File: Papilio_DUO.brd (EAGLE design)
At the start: 101.6 x 55.9 mm, 125 parts, among them IC1 FT2232H, SW1 SWITCH-2CH-6P-3010010P1, SW2 EVQQ2, T100 MOSFET-NCHANNELSMD, U1 ARDUINO_MEGA_SHIELD, U100 PCA9306, U101 ATMEGA32U4-XUMU, U2 LTC3419EMS, U3 93C46B, X1 12MHz, Y1 16MHz KX-7

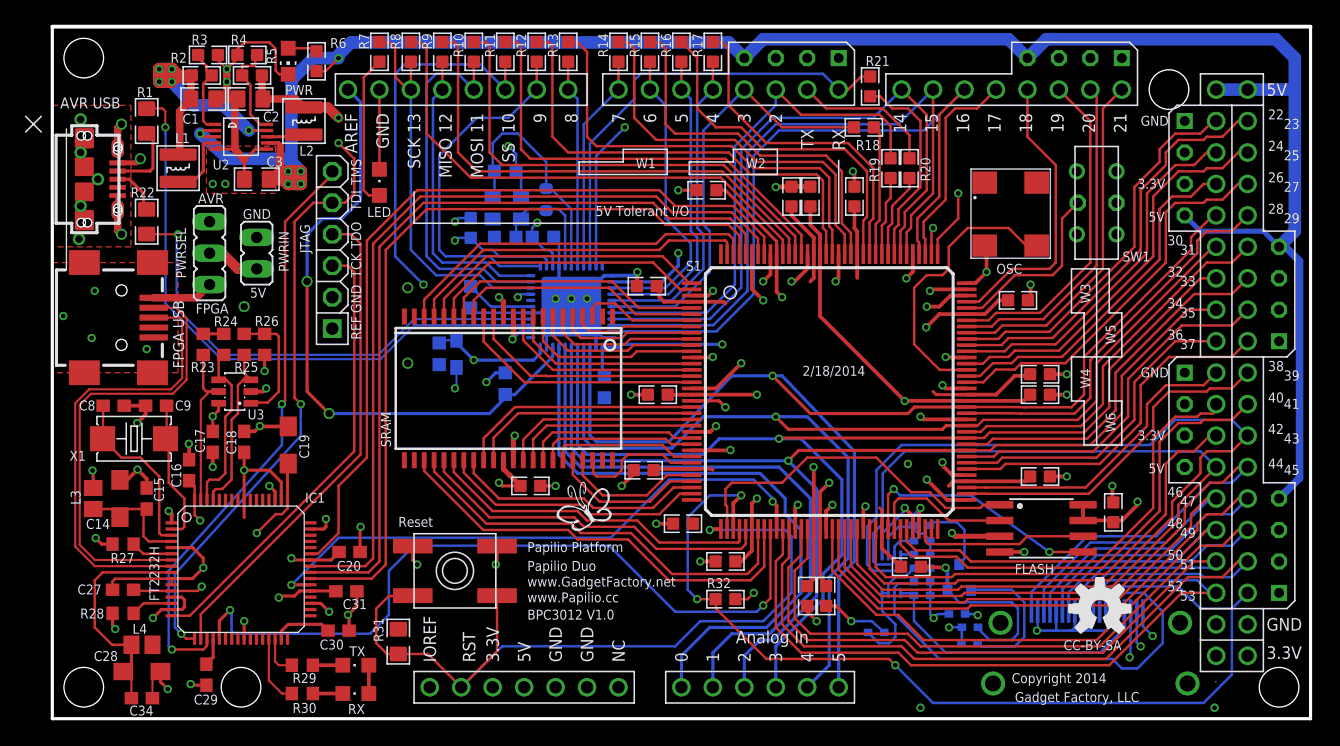
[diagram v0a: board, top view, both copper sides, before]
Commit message: Papilio DUO V1.1
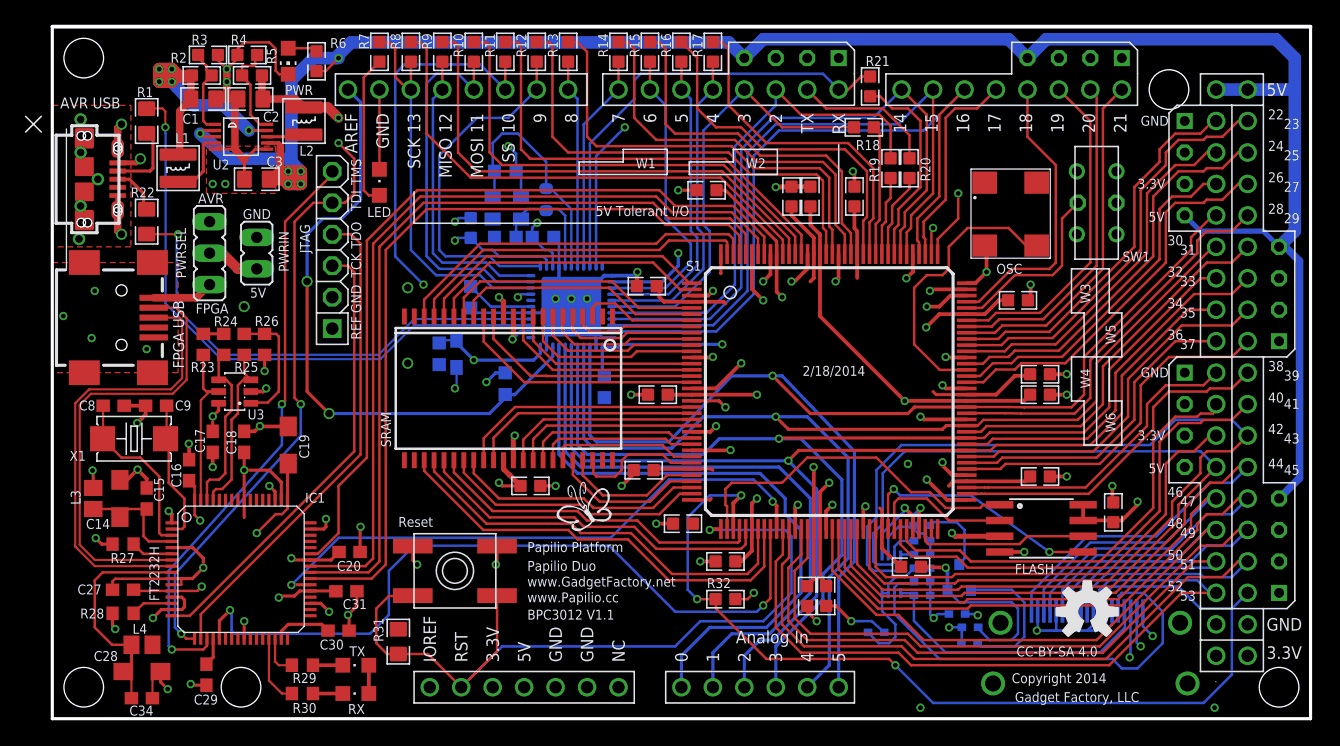
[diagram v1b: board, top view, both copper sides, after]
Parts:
- moved U$9 1.05 mm to (83.6, 8.64)
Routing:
- net 3V3: track 213.5 -> 216.7 mm
- net GND: track 237.0 -> 237.7 mm
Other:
- board text added: "BPC3012 V1.1"
- board text added: "CC-BY-SA 4.0"
- board text removed: "BPC3012 V1.0"
- board text removed: "CC-BY-SA"
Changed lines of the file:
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@@
 <setting verticaltext="up"/>
 </settings>
-<grid distance="0.05" unitdist="inch" unit="inch" style="lines" multiple="1" display="yes" altdistance="0.005" altunitdist="inch" altunit="inch"/>
+<grid distance="10" unitdist="mil" unit="mil" style="lines" multiple="1" display="yes" altdistance="1" altunitdist="mil" altunit="mil"/>
 <layers>
-<layer number="1" name="Top" color="4" fill="1" visible="yes" active="yes"/>
+<layer number="1" name="Top" color="4" fill="1" visible="no" active="yes"/>
 <layer number="2" name="Route2" color="6" fill="1" visible="no" active="yes"/>
 <layer number="3" name="Route3" color="11" fill="1" visible="no" active="yes"/>
 <layer number="14" name="Route14" color="1" fill="6" visible="no" active="no"/>
 <layer number="15" name="Route15" color="5" fill="1" visible="no" active="no"/>
-<layer number="16" name="Bottom" color="1" fill="1" visible="yes" active="yes"/>
+<layer number="16" name="Bottom" color="1" fill="1" visible="no" active="yes"/>
 <layer number="17" name="Pads" color="2" fill="1" visible="yes" active="yes"/>
 <layer number="18" name="Vias" color="2" fill="1" visible="yes" active="yes"/>
@@
 <layer number="22" name="bPlace" color="13" fill="1" visible="yes" active="yes"/>
 <layer number="23" name="tOrigins" color="15" fill="1" visible="yes" active="yes"/>
-<layer number="24" name="bOrigins" color="15" fill="1" visible="yes" active="yes"/>
+<layer number="24" name="bOrigins" color="15" fill="1" visible="no" active="yes"/>
 <layer number="25" name="tNames" color="7" fill="1" visible="yes" active="yes"/>
 <layer number="26" name="bNames" color="7" fill="1" visible="no" active="yes"/>
@@
 <layer number="29" name="tStop" color="12" fill="3" visible="no" active="yes"/>
 <layer number="30" name="bStop" color="12" fill="6" visible="no" active="yes"/>
-<layer number="31" name="tCream" color="7" fill="4" visible="no" active="yes"/>
+<layer number="31" name="tCream" color="7" fill="4" visible="yes" active="yes"/>
 <layer number="32" name="bCream" color="7" fill="5" visible="no" active="yes"/>
 <layer number="33" name="tFinish" color="6" fill="3" visible="no" active="yes"/>
@@
 <layer number="37" name="tTest" color="7" fill="1" visible="no" active="yes"/>
 <layer number="38" name="bTest" color="7" fill="1" visible="no" active="yes"/>
-<layer number="39" name="tKeepout" color="4" fill="11" visible="yes" active="yes"/>
-<layer number="40" name="bKeepout" color="1" fill="11" visible="yes" active="yes"/>
-<layer number="41" name="tRestrict" color="4" fill="10" visible="yes" active="yes"/>
-<layer number="42" name="bRestrict" color="1" fill="10" visible="yes" active="yes"/>
-<layer number="43" name="vRestrict" color="2" fill="10" visible="yes" active="yes"/>
+<layer number="39" name="tKeepout" color="4" fill="11" visible="no" active="yes"/>
+<layer number="40" name="bKeepout" color="1" fill="11" visible="no" active="yes"/>
+<layer number="41" name="tRestrict" color="4" fill="10" visible="no" active="yes"/>
+<layer number="42" name="bRestrict" color="1" fill="10" visible="no" active="yes"/>
+<layer number="43" name="vRestrict" color="2" fill="10" visible="no" active="yes"/>
 <layer number="44" name="Drills" color="7" fill="1" visible="no" active="yes"/>
 <layer number="45" name="Holes" color="7" fill="1" visible="yes" active="yes"/>
@@
 <text x="38.354" y="13.462" size="0.8" layer="130" font="vector" ratio="14">Papilio Platform</text>
 <text x="38.354" y="11.938" size="0.8" layer="130" font="vector" ratio="14">Papilio Duo</text>
-<text x="38.354" y="8.001" size="0.8" layer="130" font="vector" ratio="14">BPC3012 V1.0</text>
+<text x="38.354" y="8.001" size="0.8" layer="130" font="vector" ratio="14">BPC3012 V1.1</text>
 <text x="38.354" y="10.668" size="0.8" layer="130" font="vector" ratio="14">www.GadgetFactory.net</text>
 <text x="77.47" y="2.8702" size="0.8" layer="130" font="vector" ratio="14">Copyright 2014</text>
@@
 <text x="7.62" y="-19.05" size="2.54" layer="51" font="vector" ratio="14">Top silkscreen is on layer 130: tSilk</text>
 <text x="7.62" y="-22.86" size="2.54" layer="51" font="vector" ratio="14">Bottom silkscreen is on layer 200</text>
-<text x="81.661" y="5.5372" size="0.8" layer="130" font="vector" ratio="14">CC-BY-SA</text>
+<text x="77.851" y="5.0292" size="0.8" layer="130" font="vector" ratio="14">CC-BY-SA 4.0</text>
 </plain>
 <attributes>
@@
 <attribute name="VALUE" x="70.742" y="11.7182" size="0.05" layer="27" font="vector" ratio="0" rot="R180"/>
 </element>
-<element name="U$9" library="SparkFun-Aesthetics" package="OSHW-LOGO-M" value="" x="84.582" y="8.89"/>
+<element name="U$9" library="SparkFun-Aesthetics" package="OSHW-LOGO-M" value="" x="83.566" y="8.636"/>
 </elements>
 <signals>
@@
 <wire x1="15.49" y1="7.87" x2="15.494" y2="7.874" width="0.2032" layer="1"/>
 <via x="15.494" y="7.874" extent="1-16" drill="0.381"/>
-<wire x1="9.64" y1="11.315" x2="9.64" y2="10.815" width="0.2032" layer="1"/>
 <wire x1="9.64" y1="9.815" x2="10.45" y2="9.815" width="0.254" layer="1"/>
 <wire x1="9.64" y1="8.815" x2="10.466" y2="8.815" width="0.254" layer="1"/>
@@
 <wire x1="8.815" y1="8.815" x2="8.128" y2="8.128" width="0.254" layer="1"/>
 <via x="8.128" y="8.128" extent="1-16" drill="0.381"/>
-<wire x1="9.64" y1="11.315" x2="11.315" y2="11.315" width="0.254" layer="1"/>
+<wire x1="9.64" y1="11.315" x2="10.414" y2="11.315" width="0.254" layer="1"/>
+<wire x1="10.414" y1="11.315" x2="11.315" y2="11.315" width="0.254" layer="1"/>
 <wire x1="11.315" y1="11.315" x2="12.192" y2="12.192" width="0.254" layer="1"/>
 <via x="12.192" y="12.192" extent="1-16" drill="0.381"/>
@@
 <wire x1="62.484" y1="9.106" x2="63.284" y2="9.106" width="0.254" layer="1"/>
 <wire x1="63.284" y1="9.106" x2="64.516" y2="7.874" width="0.254" layer="1"/>
+<wire x1="9.64" y1="10.815" x2="10.414" y2="10.815" width="0.2032" layer="1"/>
+<wire x1="10.414" y1="10.815" x2="10.414" y2="11.315" width="0.2032" layer="1"/>
+<wire x1="2.286" y1="45.72" x2="2.5908" y2="46.863" width="0" layer="19" extent="1-1"/>
+<wire x1="8.188" y1="30.785" x2="7.62" y2="29.845" width="0" layer="19" extent="1-1"/>
+<wire x1="2.5908" y1="44.577" x2="2.286" y2="45.72" width="0" layer="19" extent="1-1"/>
+<wire x1="2.5908" y1="42.545" x2="2.286" y2="41.402" width="0" layer="19" extent="1-1"/>
+<wire x1="2.5908" y1="40.259" x2="2.286" y2="41.402" width="0" layer="19" extent="1-1"/>
 </signal>
 <signal name="OSC_IN">
@@
 <wire x1="85.8138" y1="16.002" x2="85.6742" y2="15.8624" width="0.3048" layer="1"/>
 <wire x1="12.192" y1="31.076" x2="13.843" y2="31.076" width="0.254" layer="1"/>
+<wire x1="53.988" y1="37.516" x2="53.988" y2="35.954" width="0.254" layer="1"/>
+<wire x1="53.988" y1="35.954" x2="53.975" y2="35.941" width="0.254" layer="1"/>
+<wire x1="51.638" y1="17.666" x2="53.099" y2="17.666" width="0.254" layer="1"/>
+<wire x1="53.099" y1="17.666" x2="53.213" y2="17.78" width="0.254" layer="1"/>
 </signal>
 <signal name="1V2">
